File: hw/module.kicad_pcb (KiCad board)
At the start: 2 copper layers, 30 x 30 mm, 35 parts, among them U1 CFPS-39, U2 CFPS-39, U3 74LVC1G125, U4 74 LVC 1G3157GW,125, U5 MAX919, U6 TSSOP20, U7 BAS70-7-F

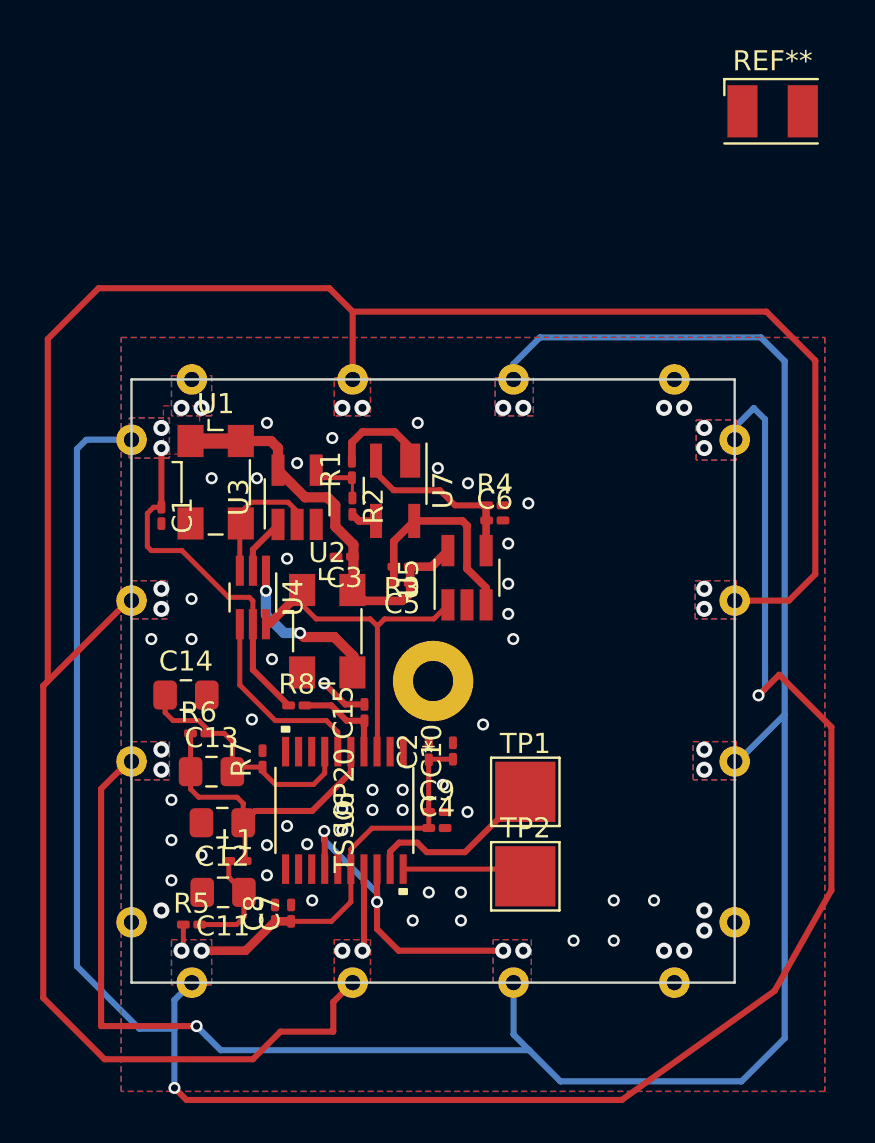
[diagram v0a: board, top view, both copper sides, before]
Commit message: Footprint fix, and first PCB release
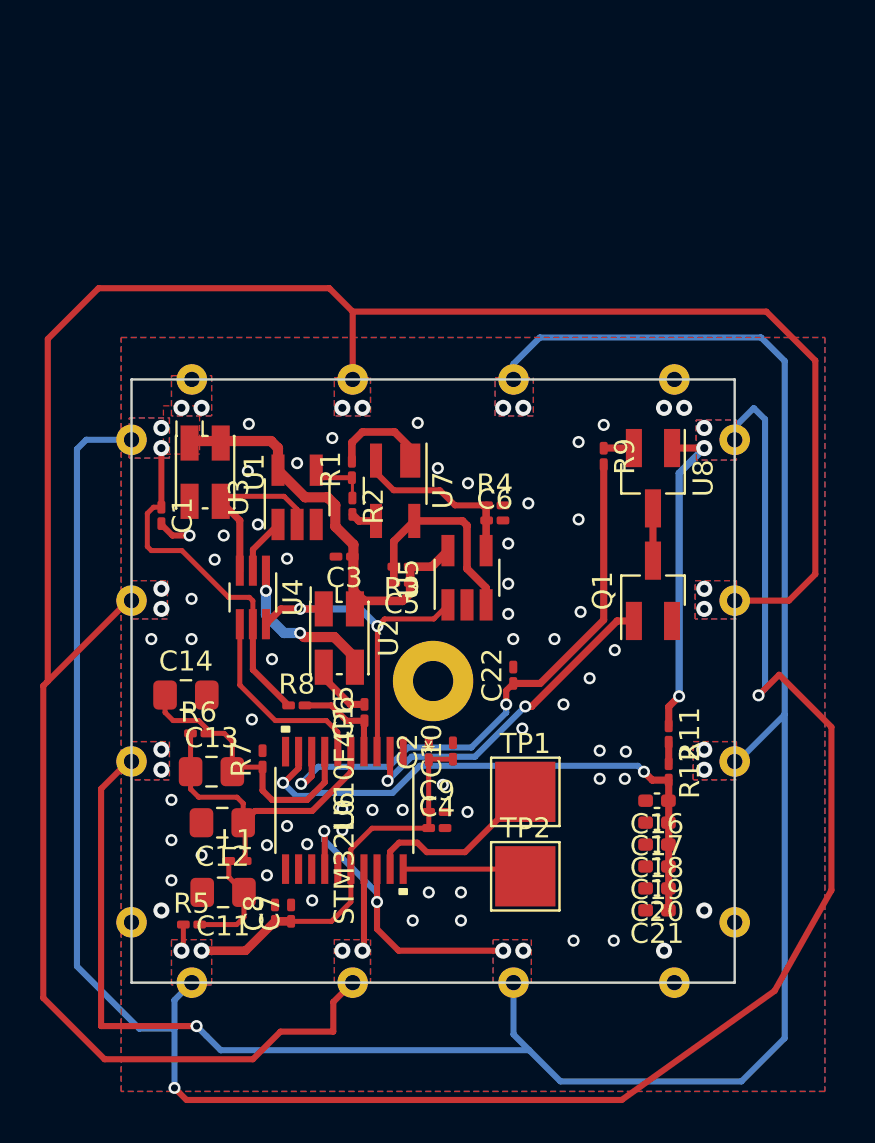
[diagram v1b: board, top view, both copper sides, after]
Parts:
- removed REF**: LED_PLCC-2, LED_SMD:LED_PLCC-2
- added C16: 4u7, Capacitor_SMD:C_0402_1005Metric_Pad0.74x0.62mm_HandSolder, F.Cu at (69.2, 63.0)
- added C17: 4u7, Capacitor_SMD:C_0402_1005Metric_Pad0.74x0.62mm_HandSolder, F.Cu at (69.2, 64.1)
- added C18: 4u7, Capacitor_SMD:C_0402_1005Metric_Pad0.74x0.62mm_HandSolder, F.Cu at (69.2, 65.2)
- added C19: 4u7, Capacitor_SMD:C_0402_1005Metric_Pad0.74x0.62mm_HandSolder, F.Cu at (69.2, 66.3)
- added C20: 4u7, Capacitor_SMD:C_0402_1005Metric_Pad0.74x0.62mm_HandSolder, F.Cu at (69.2, 67.4)
- added C21: 4u7, Capacitor_SMD:C_0402_1005Metric_Pad0.74x0.62mm_HandSolder, F.Cu at (69.2, 68.5)
- added C22: 200p, Capacitor_SMD:C_0201_0603Metric_Pad0.64x0.40mm_HandSolder, F.Cu at (62.0, 56.8)
- added Q1: MUN 2211, Package_TO_SOT_SMD:SOT-23_Handsoldering, F.Cu at (69.0, 52.6)
- added R11: 150k, Resistor_SMD:R_0201_0603Metric_Pad0.64x0.40mm_HandSolder, F.Cu at (69.7, 59.7)
- added R12: 150k, Resistor_SMD:R_0201_0603Metric_Pad0.64x0.40mm_HandSolder, F.Cu at (69.7, 61.6)
- added R9: 100, Resistor_SMD:R_0201_0603Metric_Pad0.64x0.40mm_HandSolder, F.Cu at (66.5, 45.9)
- added U8: SS39ET, Package_TO_SOT_SMD:SOT-23_Handsoldering, F.Cu at (69.0, 47.0)
- L1: value L -> 27n
- R5: value R -> 10
- U1, U2: footprint Oscillator:Oscillator_SMD_Fox_FT5H_5.0x3.2mm -> Oscillator:Oscillator_SMD_EuroQuartz_XO32-4Pin_3.2x2.5mm_HandSoldering
- U6: value TSSOP20 -> STM32L010F4P6
- moved U1 0.73 mm to (46.7, 46.7), turned to -90 degrees
- moved U2 0.69 mm to (53.4, 55.0), turned to -90 degrees
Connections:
- U6 pad 2: unconnected-(U6-Pad2) -> /hall_on
- U6 pad 8: unconnected-(U6-Pad8) -> /hall_exp
- U6 pad 9: unconnected-(U6-Pad9) -> /Cap_experiment
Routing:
- net /Cap_experiment: track 0.00 -> 28.7 mm, vias 0 -> 2
- net /hall_exp: track 0.00 -> 28.7 mm, vias 0 -> 2
- net /hall_on: track 0.00 -> 17.0 mm, vias 0 -> 2
- net +3.3V: track 167.4 -> 183.6 mm, vias 10 -> 11
- net Net-(Q1-Pad3): track 0.00 -> 2.60 mm
- net GND: track 5.25 -> 7.59 mm, vias 53 -> 61
- net Net-(U1-Pad3): track 6.77 -> 8.77 mm
- net Net-(R9-Pad1): track 0.00 -> 1.50 mm
- net /half_vref: track 12.9 -> 14.4 mm
- net Net-(R11-Pad2): track 0.00 -> 1.07 mm
- net /OSC_STAT: track 17.5 -> 17.6 mm, vias 0 -> 2
